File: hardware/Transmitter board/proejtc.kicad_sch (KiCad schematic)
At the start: 4 parts, among them U1 PAM8403D, U2 MAX4466EXK_T

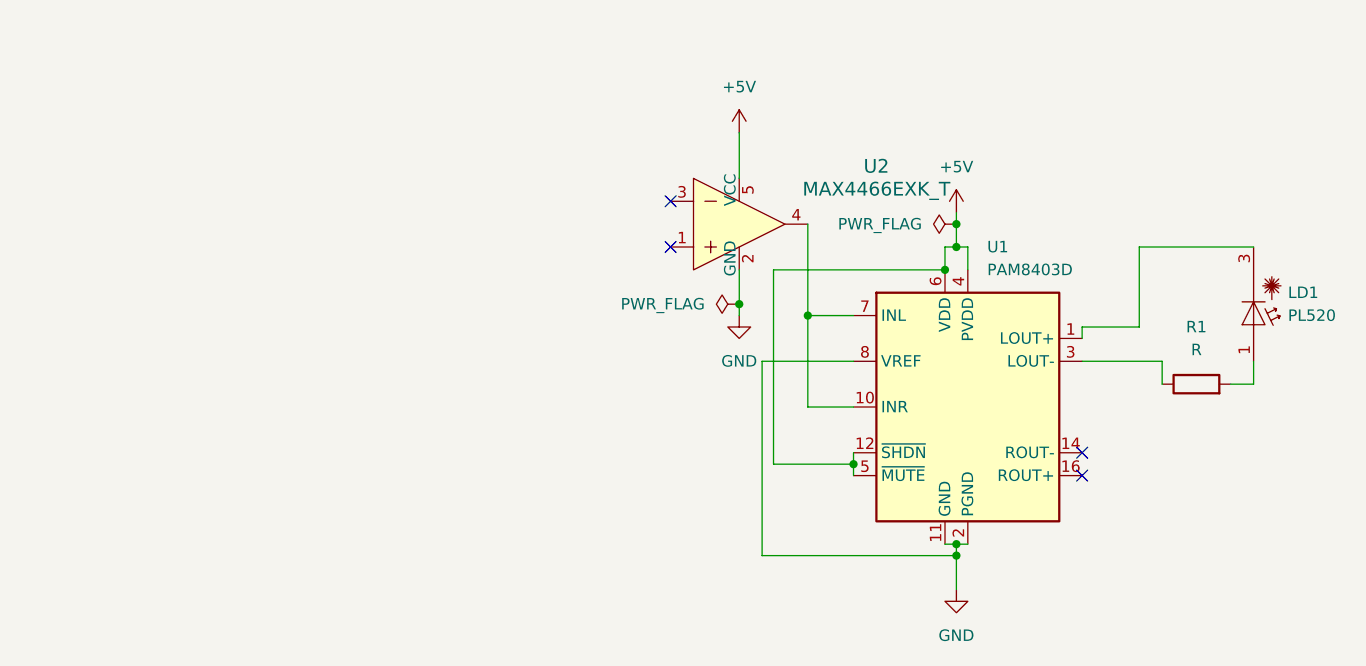
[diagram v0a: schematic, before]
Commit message: Add files via upload
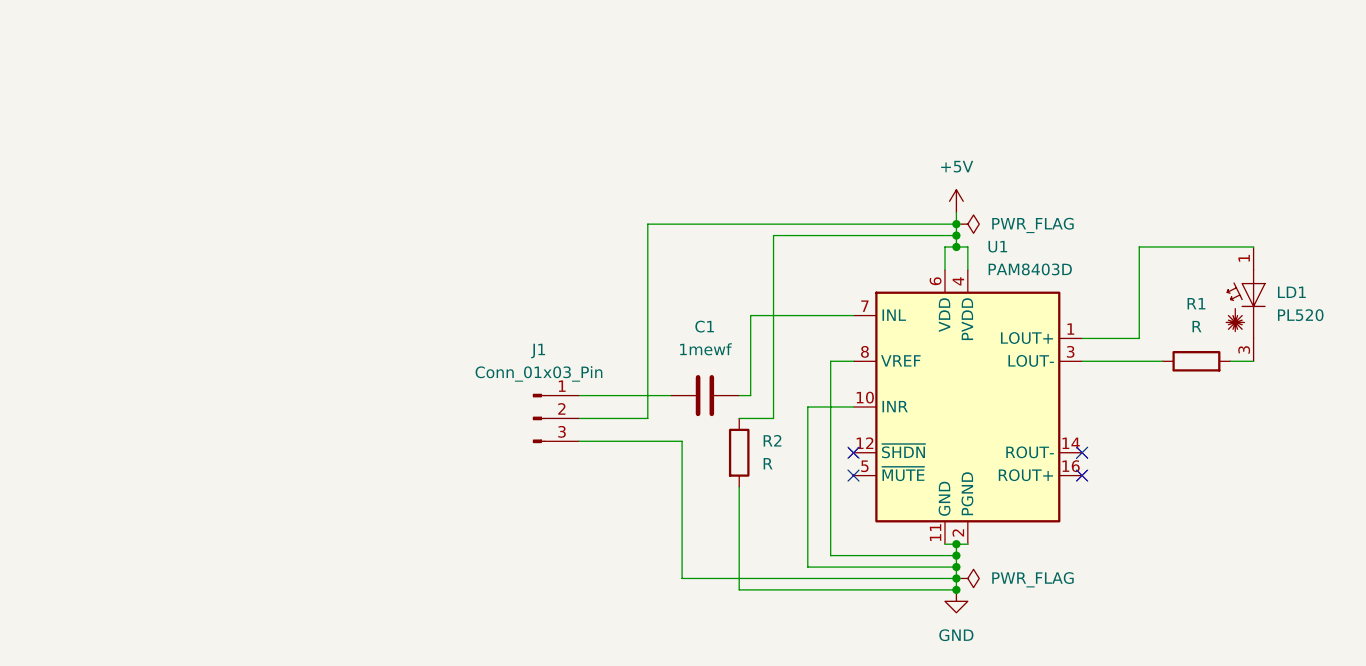
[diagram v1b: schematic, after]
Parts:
- removed U2: MAX4466EXK_T, digikey-footprints:SOT-353, symbol dk_Linear-Amplifiers-Audio:MAX4466EXK_T
- added C1: 1mewf, symbol Device:C
- added J1: Conn_01x03_Pin, Connector_PinSocket_2.54mm:PinSocket_1x03_P2.54mm_Horizontal, symbol Connector:Conn_01x03_Pin
- added R2: R, symbol Device:R
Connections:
- net +5V: now also J1.2 (Pin_2), R2.1; no longer U1.12 (~{SHDN}), U1.5 (~{MUTE})
- net GND: now also U1.10 (INR), J1.3 (Pin_3), R2.2
- net at U1.7 (INL): now also C1.1; no longer U1.10 (INR)
- net at LD1.1 (A): now also U1.1 (LOUT+); no longer R1.2
- net at LD1.3 (C): now also R1.2; no longer U1.1 (LOUT+)
- new net: C1.2, J1.1 (Pin_1)
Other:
- moved on the sheet: LD1, R1

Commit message: Add files via upload
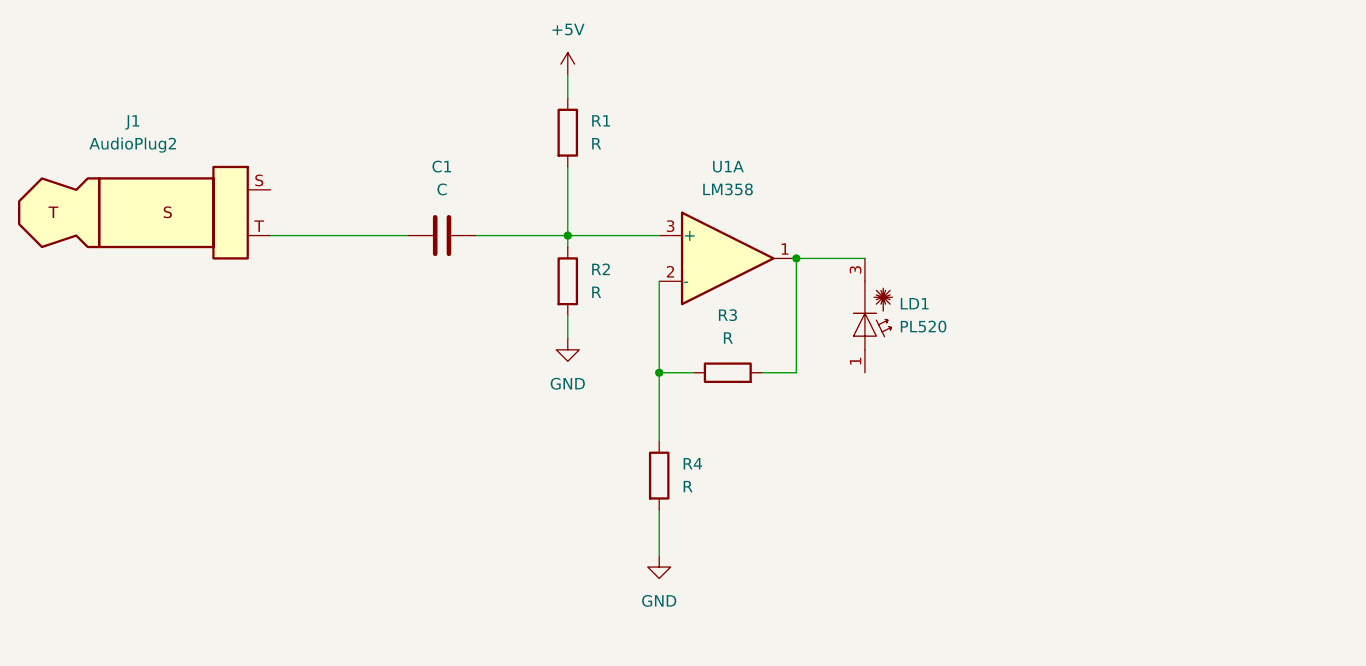
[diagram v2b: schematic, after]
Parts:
- removed J1: Conn_01x03_Pin, Connector_PinSocket_2.54mm:PinSocket_1x03_P2.54mm_Horizontal, symbol Connector:Conn_01x03_Pin
- removed U1: PAM8403D, Package_SO:SOIC-16_3.9x9.9mm_P1.27mm, symbol Amplifier_Audio:PAM8403D
- added J1: AudioPlug2, symbol Connector_Audio:AudioPlug2
- added R3, R4: R, symbol Device:R
- added U1: LM358, symbol Amplifier_Operational:LM358
- C1: value 1mewf -> C
- R1: footprint Resistor_THT:R_Axial_DIN0204_L3.6mm_D1.6mm_P5.08mm_Vertical -> (none)
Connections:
- net +5V: now also R1.1; no longer R2.1
- net GND: now also R4.2
- net at C1.1: now also J1.T
- net at C1.2: now also R1.2, R2.1, U1.3 (+)
- net at LD1.3 (C): now also R3.2, U1.1; no longer R1.2
- new net: R3.1, R4.1, U1.2 (-)
- no-connect marks 4 -> 0
